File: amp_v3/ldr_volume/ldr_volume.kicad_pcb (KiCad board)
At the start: 2 copper layers, 424.2 x 159 mm, 175 parts, among them J1 A_IN, J10 CTRL, J13 NTC, J14 Conn_01x05_Pin, J15 PWR_IN, J16 CTRL, J17 CTRL, J18 PWR3, J19 PWR_IN, J2 A_OUT, J20 I2C_L, J21 I2C_R, J22 PWR_SEL, J23 MUTE, J24 UART, J25 PWR4, J26 Conn_01x03_Pin, J27 5V_IN, J28 5V_IN, J29 IR, J3 5v_in, J30 TFT, J31 S_AIN_L, J32 S_AIN_R, J33 IR_SENSOR, J34 I2C, J35 BTN_VOL, J36 MUTE, J38 BTN_MENU, J39 UART, J4 ADS1115, J40 BTN_EXT1, J41 BTN_EXT2, J42 PWR_BTN, J43 PWR_BTN_LED, J44 PWR_RLY, J45 MUTE_OUT, J46 ALPS, J47 MUTE, J5 I2C_R, J6 PWR1, J7 PWR2, J8 PWR3, J9 PWR4, K1 G5V-2, Q1 BC547, Q10 BC557, Q11 2N7000, Q12 2N7000, Q13 BC547, Q14 BC547, Q2 BC557, Q3 BC547, Q4 BC557, Q5 BC547, Q6 BC557, Q7 BC547, Q8 BC557, Q9 BC547, SW1 SW_UP, SW2 SW_DN, SW3 SW_LT, SW4 SW_RT, SW5 SW_PWR, U1 MCP1700x-330xxTO, U2 NSL-32-SR3-Rseries, U3 NSL-32-SR3-Rshunt, U4 4N25, U5 NSL-32-SR3, U6 TSOP312xx, U7 IRM-10-5

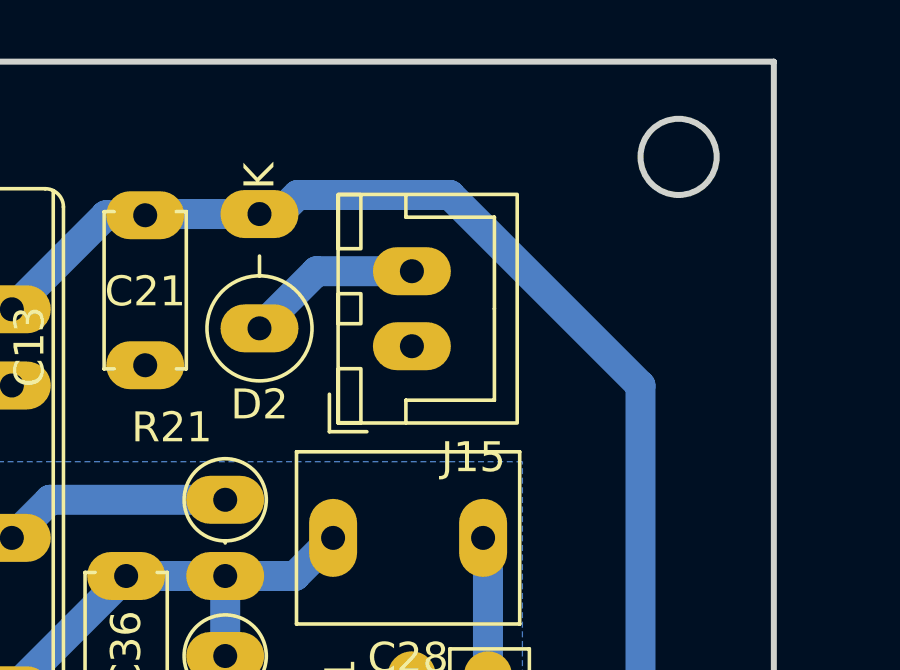
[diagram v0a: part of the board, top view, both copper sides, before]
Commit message: updates
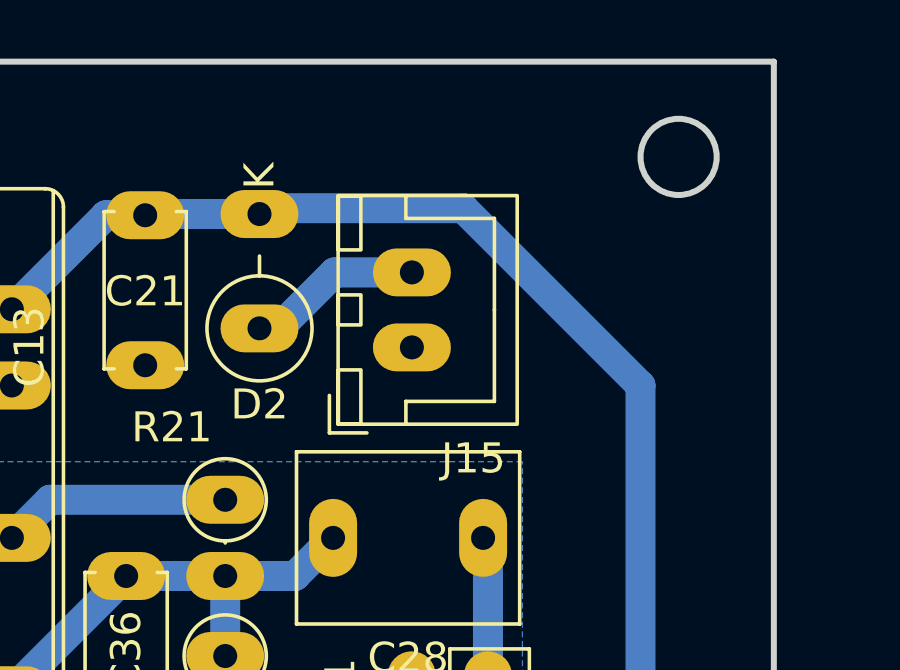
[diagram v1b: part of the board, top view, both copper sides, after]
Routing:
- net /Main Board/5v_local: track 118.0 -> 118.6 mm
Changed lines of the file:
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@@
 	(footprint "Connector_JST:JST_XH_B2B-XH-A_1x02_P2.50mm_Vertical"
 		(layer "F.Cu")
-		(at 76.748028 -74.3744 90)
+		(at 76.748028 -74.3344 90)
 		(descr "JST XH series connector, B2B-XH-A (http://www.jst-mfg.com/product/pdf/eng/eXH.pdf)")
 		(tags "connector JST XH vertical")
@@
 	)
 	(segment
-		(start 72.938028 -79.4144)
-		(end 78.018028 -79.4144)
-		(width 1)
-		(layer "B.Cu")
-		(net "/Main Board/5v_local")
-	)
-	(segment
-		(start 72.498028 -78.9744)
-		(end 72.938028 -79.4144)
-		(width 1)
-		(layer "B.Cu")
-		(net "/Main Board/5v_local")
-	)
-	(segment
 		(start 58.303028 -75.6044)
 		(end 48.203028 -65.5044)
@@
 	)
 	(segment
+		(start 71.668028 -78.7794)
+		(end 71.863028 -78.9744)
+		(width 1)
+		(layer "B.Cu")
+		(net "/Main Board/5v_local")
+	)
+	(segment
 		(start 33.568028 -63.834248)
 		(end 33.568028 -57.8244)
@@
 	)
 	(segment
+		(start 71.863028 -78.9744)
+		(end 78.458028 -78.9744)
+		(width 1)
+		(layer "B.Cu")
+		(net "/Main Board/5v_local")
+	)
+	(segment
 		(start 59.603028 -75.6044)
 		(end 58.303028 -75.6044)
@@
 	)
 	(segment
-		(start 78.018028 -79.4144)
-		(end 84.368028 -73.0644)
-		(width 1)
-		(layer "B.Cu")
-		(net "/Main Board/5v_local")
-	)
-	(segment
 		(start 84.368028 -34.3294)
 		(end 77.383028 -27.3444)
@@
 	)
 	(segment
+		(start 78.458028 -78.9744)
+		(end 84.368028 -73.0644)
+		(width 1)
+		(layer "B.Cu")
+		(net "/Main Board/5v_local")
+	)
+	(segment
 		(start 137.346728 -152.9108)
 		(end 134.791328 -150.3554)
@@
 	)
 	(segment
-		(start 76.748028 -76.8744)
-		(end 73.573028 -76.8744)
+		(start 76.748028 -76.8344)
+		(end 74.168028 -76.8344)
+		(width 1)
+		(layer "B.Cu")
+		(net "/Main Board/5V_board1")
+	)
+	(segment
+		(start 74.168028 -76.8344)
+		(end 72.303028 -74.9694)
 		(width 1)
 		(layer "B.Cu")
@@
 	)
 	(segment
-		(start 73.573028 -76.8744)
+		(start 72.303028 -74.9694)
 		(end 71.668028 -74.9694)
 		(width 1)
@@
 	)
 	(segment
+		(start 177.078028 -134.6394)
+		(end 177.078028 -137.9614)
+		(width 1)
+		(layer "B.Cu")
+		(net "/LDR Driver/MUTE_CTRL")
+	)
+	(segment
+		(start 177.078028 -137.9614)
+		(end 174.792028 -140.2474)
+		(width 1)
+		(layer "B.Cu")
+		(net "/LDR Driver/MUTE_CTRL")
+	)
+	(segment
+		(start 144.693028 -130.2144)
+		(end 144.693028 -133.0284)
+		(width 1)
+		(layer "B.Cu")
+		(net "/LDR Driver/MUTE_CTRL")
+	)
+	(segment
+		(start 139.768828 -130.0508)
+		(end 144.529428 -130.0508)
+		(width 1)
+		(layer "B.Cu")
+		(net "/LDR Driver/MUTE_CTRL")
+	)
+	(segment
+		(start 144.693028 -133.0284)
+		(end 146.979028 -135.3144)
+		(width 1)
+		(layer "B.Cu")
+		(net "/LDR Driver/MUTE_CTRL")
+	)
+	(segment
 		(start 40.453028 -75.6044)
 		(end 38.053028 -78.0044)
@@
 	)
 	(segment
-		(start 177.078028 -134.6394)
-		(end 177.078028 -137.9614)
-		(width 1)
-		(layer "B.Cu")
-		(net "/LDR Driver/MUTE_CTRL")
-	)
-	(segment
-		(start 177.078028 -137.9614)
-		(end 174.792028 -140.2474)
-		(width 1)
-		(layer "B.Cu")
-		(net "/LDR Driver/MUTE_CTRL")
-	)
-	(segment
-		(start 144.693028 -130.2144)
-		(end 144.693028 -133.0284)
-		(width 1)
-		(layer "B.Cu")
-		(net "/LDR Driver/MUTE_CTRL")
-	)
-	(segment
-		(start 139.768828 -130.0508)
-		(end 144.529428 -130.0508)
-		(width 1)
-		(layer "B.Cu")
-		(net "/LDR Driver/MUTE_CTRL")
-	)
-	(segment
-		(start 144.693028 -133.0284)
-		(end 146.979028 -135.3144)
-		(width 1)
-		(layer "B.Cu")
-		(net "/LDR Driver/MUTE_CTRL")
-	)
-	(segment
